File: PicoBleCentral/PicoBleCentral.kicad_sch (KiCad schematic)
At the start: 10 parts, among them IC2 VREG-OKI-78SR-3.3/1.5-W36, J5 Sel Vreg In, Q3 DMG2305UX-7, U2 R-78E5.0-1.0

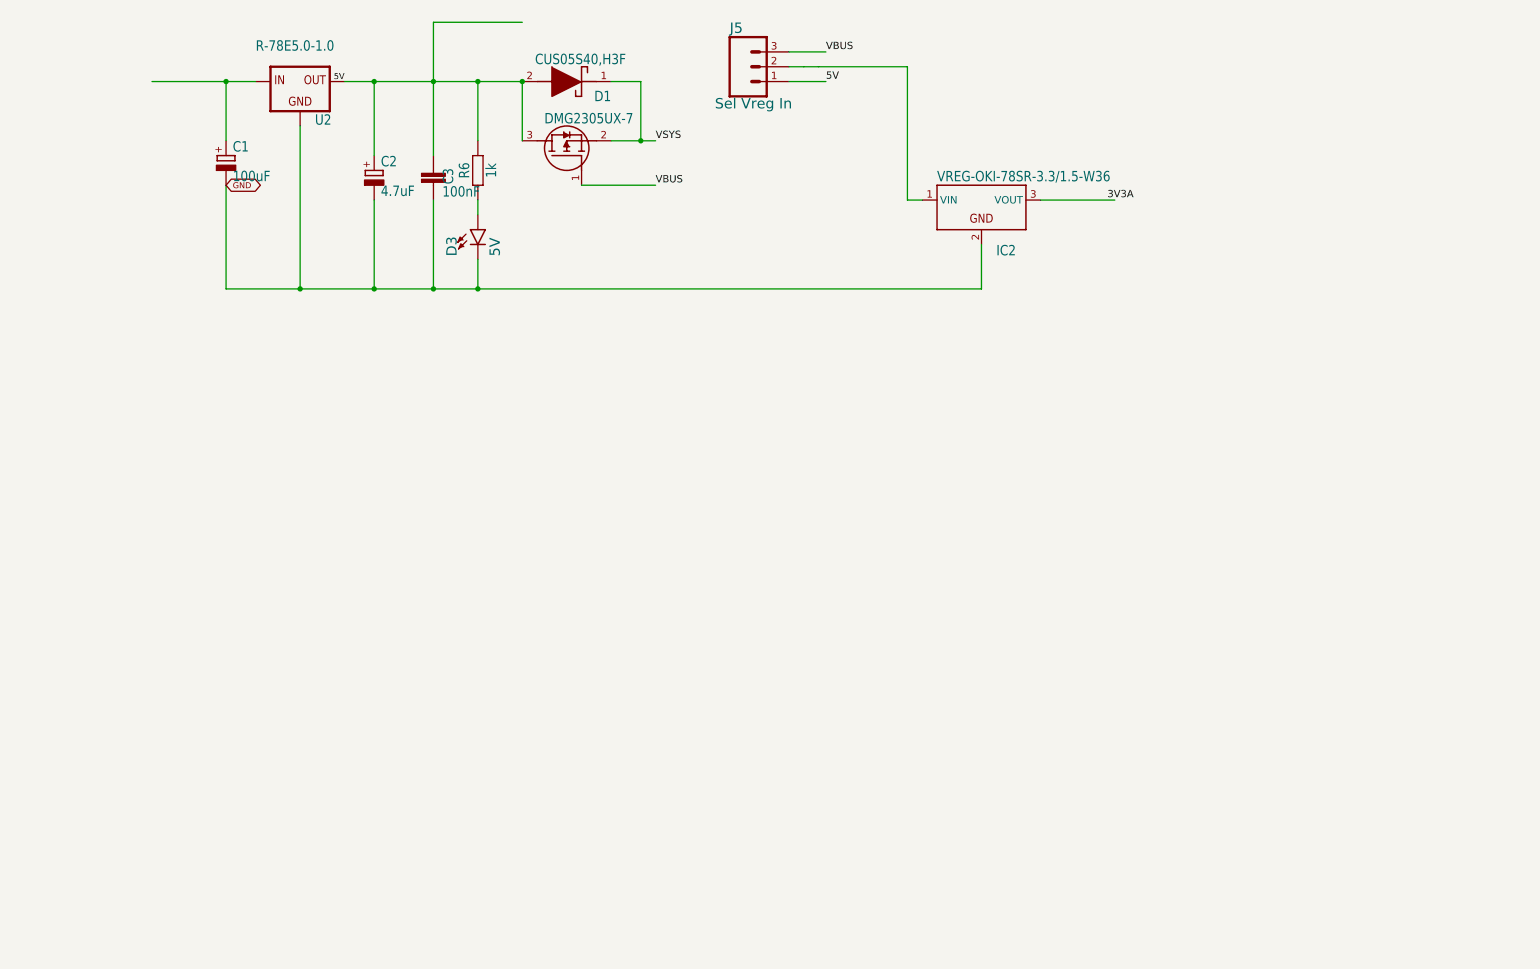
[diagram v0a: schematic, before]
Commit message: 26/05/25 20:18 Titan.local
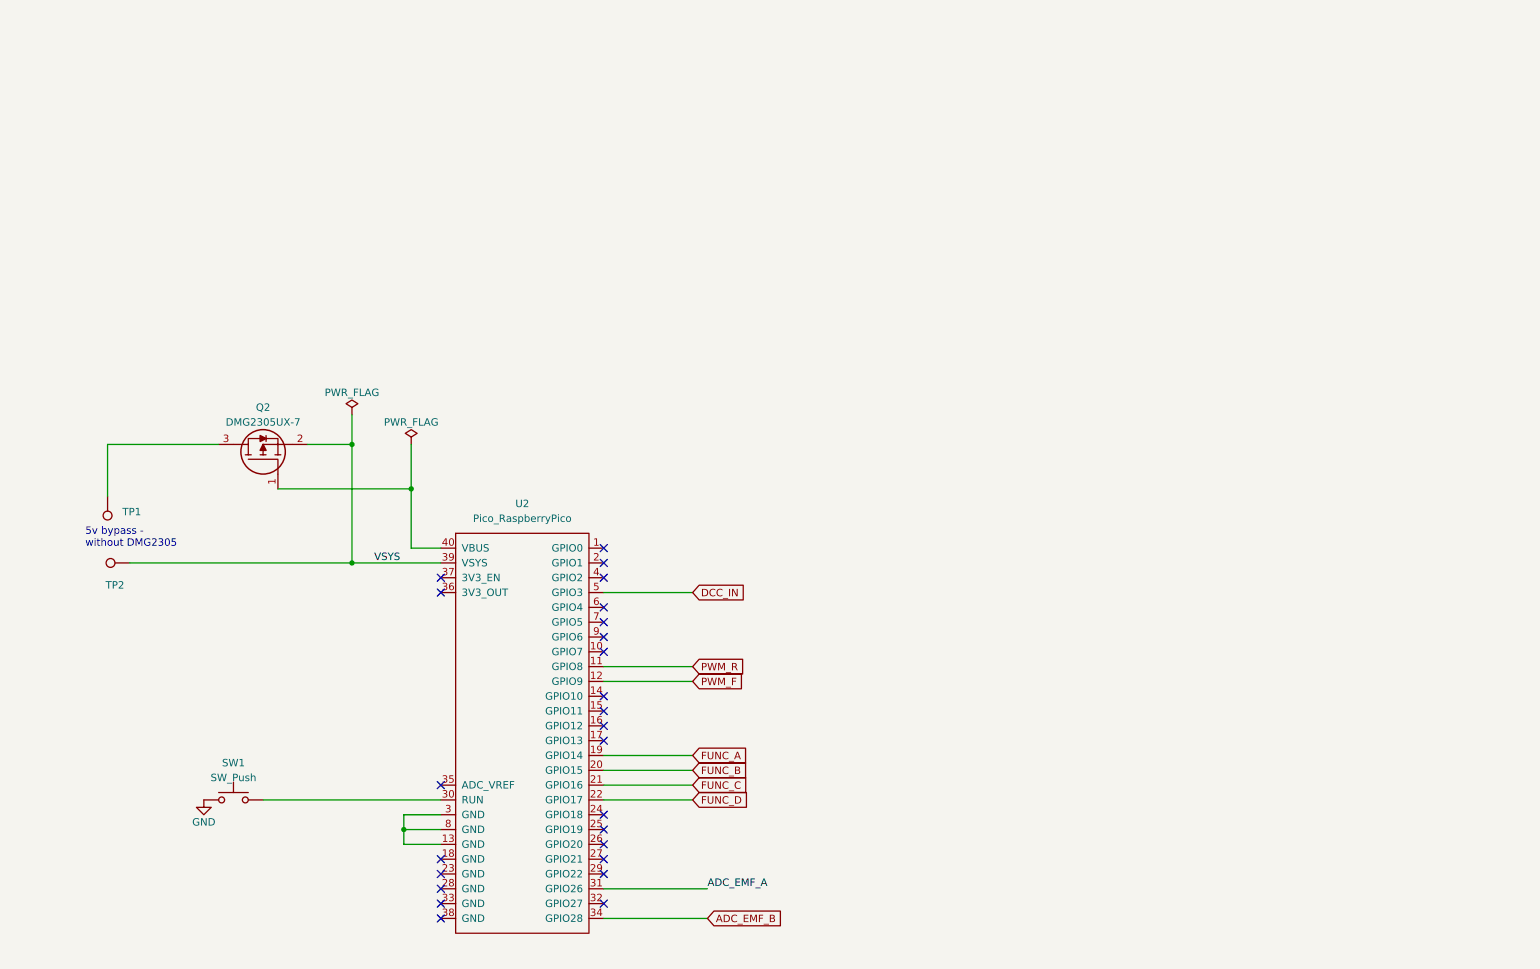
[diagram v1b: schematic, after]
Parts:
- removed C1: 100uF, PicoCanSmd31:E5-8,5, symbol PicoCanSmd31-eagle-import:CPOL-EUE5-8.5
- removed C2: 4.7uF, PicoCanSmd31:E5-8,5, symbol PicoCanSmd31-eagle-import:CPOL-EUE5-8.5
- removed C3: 100nF, PicoCanSmd31:C025-024X044, symbol PicoCanSmd31-eagle-import:C-EU025-024X044
- removed D1: CUS05S40,H3F, PicoCanSmd31:1SS357TPH3F, symbol PicoCanSmd31-eagle-import:CUS05S40,H3F
- removed D3: 5V, PicoCanSmd31:LED_3MM, symbol PicoCanSmd31-eagle-import:LED3MM
- removed IC2: VREG-OKI-78SR-3.3/1.5-W36, PicoCanSmd31:OKI-78SR, symbol PicoCanSmd31-eagle-import:VREG-OKI-78SR-3.3/1.5-W36
- removed J5: Sel Vreg In, PicoCanSmd31:1X03, symbol PicoCanSmd31-eagle-import:CONN_03
- removed Q3: DMG2305UX-7, PicoCanSmd31:SOT96P240X110-3N, symbol PicoCanSmd31-eagle-import:DMG2305UX-7
- removed R6: 1k, PicoCanSmd31:C1206, symbol PicoCanSmd31-eagle-import:RESISTOR-1206
- removed U2: R-78E5.0-1.0, PicoCanSmd31:DC-DC_CONVERTER_78XX, symbol PicoCanSmd31-eagle-import:R-78E5.0-1.0
- added Q2: DMG2305UX-7, Package_TO_SOT_SMD:SOT-23-3, symbol DMG2305UX-7:DMG2305UX-7
- added SW1: SW_Push, Button_Switch_SMD:SW_Tactile_SPST_NO_Straight_CK_PTS636Sx25SMTRLFS, symbol Switch:SW_Push
- added TP1, TP2: TestPoint, TestPoint:TestPoint_Pad_2.0x2.0mm, symbol Connector:TestPoint
- added U2: Pico_RaspberryPico, PicoNoSwd:RaspberryPico_TH_NoSWD, symbol PicoNoSwd:RaspberryPico-Pico
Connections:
- net GND: now also SW1.2
- net VSYS: now also Q2.2, TP2.1, U2.39 (VSYS)
- new net: Q2.1, U2.40 (VBUS)
- new net: Q2.3, TP1.1
- new net: SW1.1, U2.30 (RUN)
- new net: U2.13 (GND), U2.3 (GND), U2.8 (GND)
- new net ADC_EMF_A: U2.31 (GPIO26)
- new net ADC_EMF_B: U2.34 (GPIO28)
- new net DCC_IN: U2.5 (GPIO3)
- new net FUNC_A: U2.19 (GPIO14)
- new net FUNC_B: U2.20 (GPIO15)
- new net FUNC_C: U2.21 (GPIO16)
- new net FUNC_D: U2.22 (GPIO17)
- new net PWM_F: U2.12 (GPIO9)
- new net PWM_R: U2.11 (GPIO8)
- no-connect marks 0 -> 25
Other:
- note added: "5v bypass - without DMG2305"

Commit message: 26/05/25 20:40 Titan.local
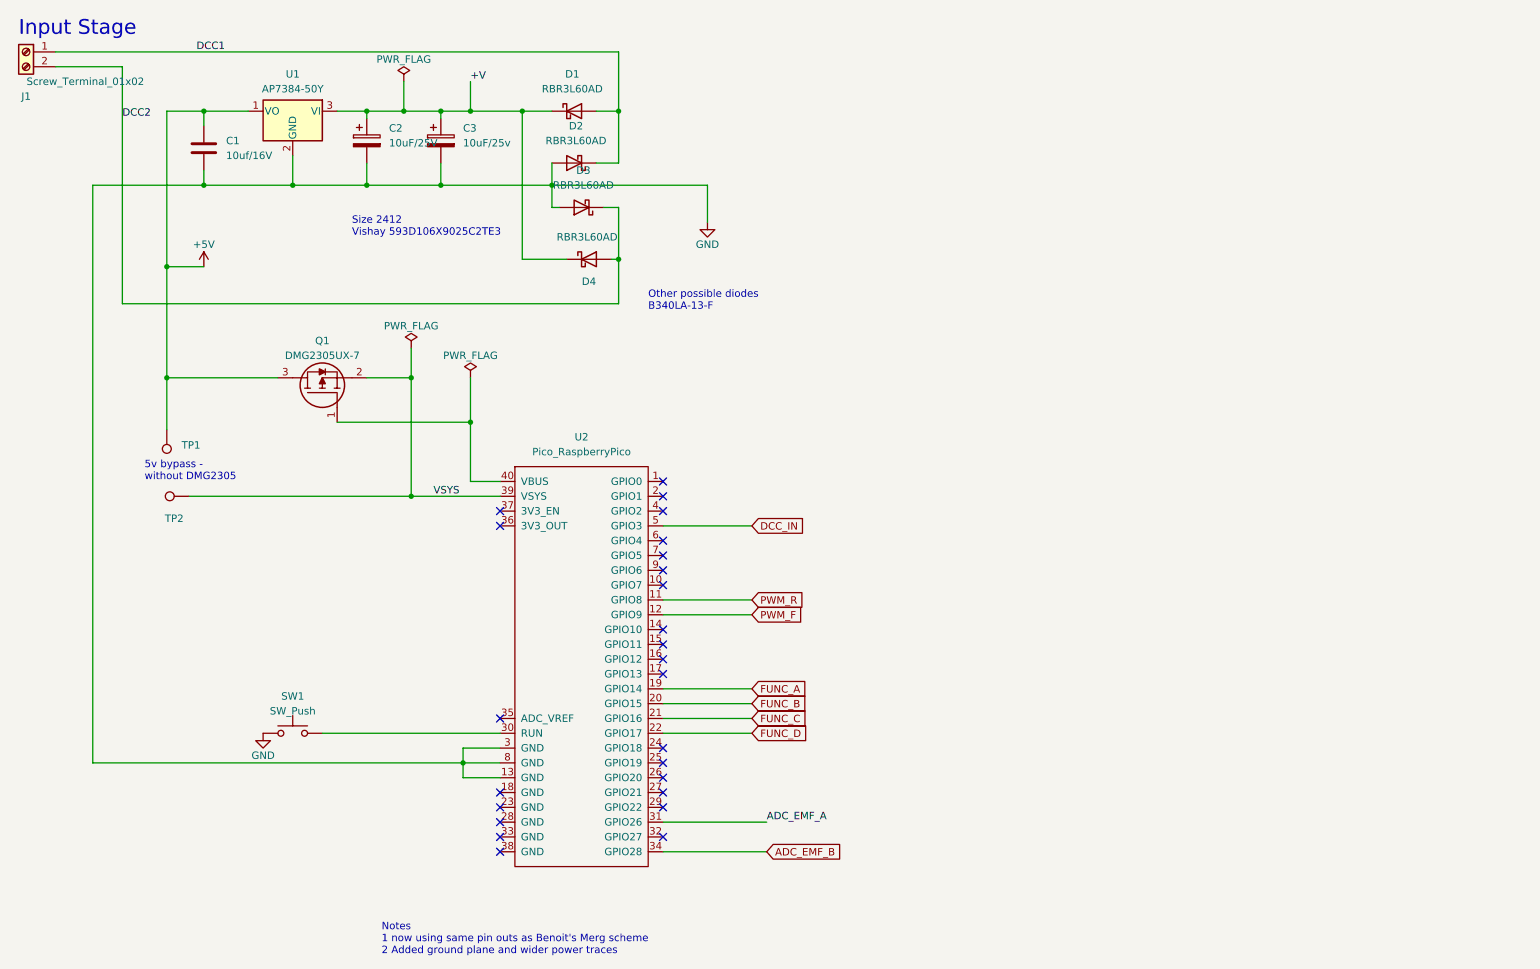
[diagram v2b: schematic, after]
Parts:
- removed Q2: DMG2305UX-7, Package_TO_SOT_SMD:SOT-23-3, symbol DMG2305UX-7:DMG2305UX-7
- added C1: 10uf/16V, Capacitor_SMD:C_1206_3216Metric_Pad1.33x1.80mm_HandSolder, symbol Device:C
- added C2: 10uF/25V, Capacitor_Tantalum_SMD:CP_EIA-6032-20_AVX-F_Pad2.25x2.35mm_HandSolder, symbol Device:C_Polarized
- added C3: 10uF/25v, Capacitor_Tantalum_SMD:CP_EIA-6032-20_AVX-F_Pad2.25x2.35mm_HandSolder, symbol Device:C_Polarized
- added D1, D2, D3, D4: RBR3L60AD, Diode_SMD:D_SMA_Handsoldering, symbol Device:D_Schottky
- added J1: Screw_Terminal_01x02, TerminalBlock_Phoenix:TerminalBlock_Phoenix_PT-1,5-2-3.5-H_1x02_P3.50mm_Horizontal, symbol Connector:Screw_Terminal_01x02
- added Q1: DMG2305UX-7, Package_TO_SOT_SMD:SOT-23-3, symbol DMG2305UX-7:DMG2305UX-7
- added U1: AP7384-50Y, Package_TO_SOT_SMD:SOT-89-3, symbol Regulator_Linear:AP7384-50Y
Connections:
- net GND: now also U2.13 (GND), U2.3 (GND), U2.8 (GND), C1.2, C2.2, C3.2, D2.2 (A), D3.2 (A), U1.2 (GND)
- net VSYS: now also Q1.2
- net at U2.40 (VBUS): now also Q1.1
- net +5V: now reaches TP1.1
- net +5V: now also C1.1, Q1.3, U1.1 (VO)
- new net +V: C2.1, C3.1, D1.1 (K), D4.1 (K), U1.3 (VI)
- new net DCC1: D1.2 (A), D2.1 (K), J1.1 (Pin_1)
- new net DCC2: D3.1 (K), D4.2 (A), J1.2 (Pin_2)
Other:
- note added: "Input Stage"
- note added: "Notes 1 now using same pin outs as Benoit's Merg scheme 2 Added ground plane and wider power traces"
- note added: "Other possible diodes B340LA-13-F"
- note added: "Size 2412 Vishay 593D106X9025C2TE3"
- title: (none) -> DCC Decoder 4a - modified PCB - As 4 but with ground plane

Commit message: 26/05/25 22:33 Titan.local
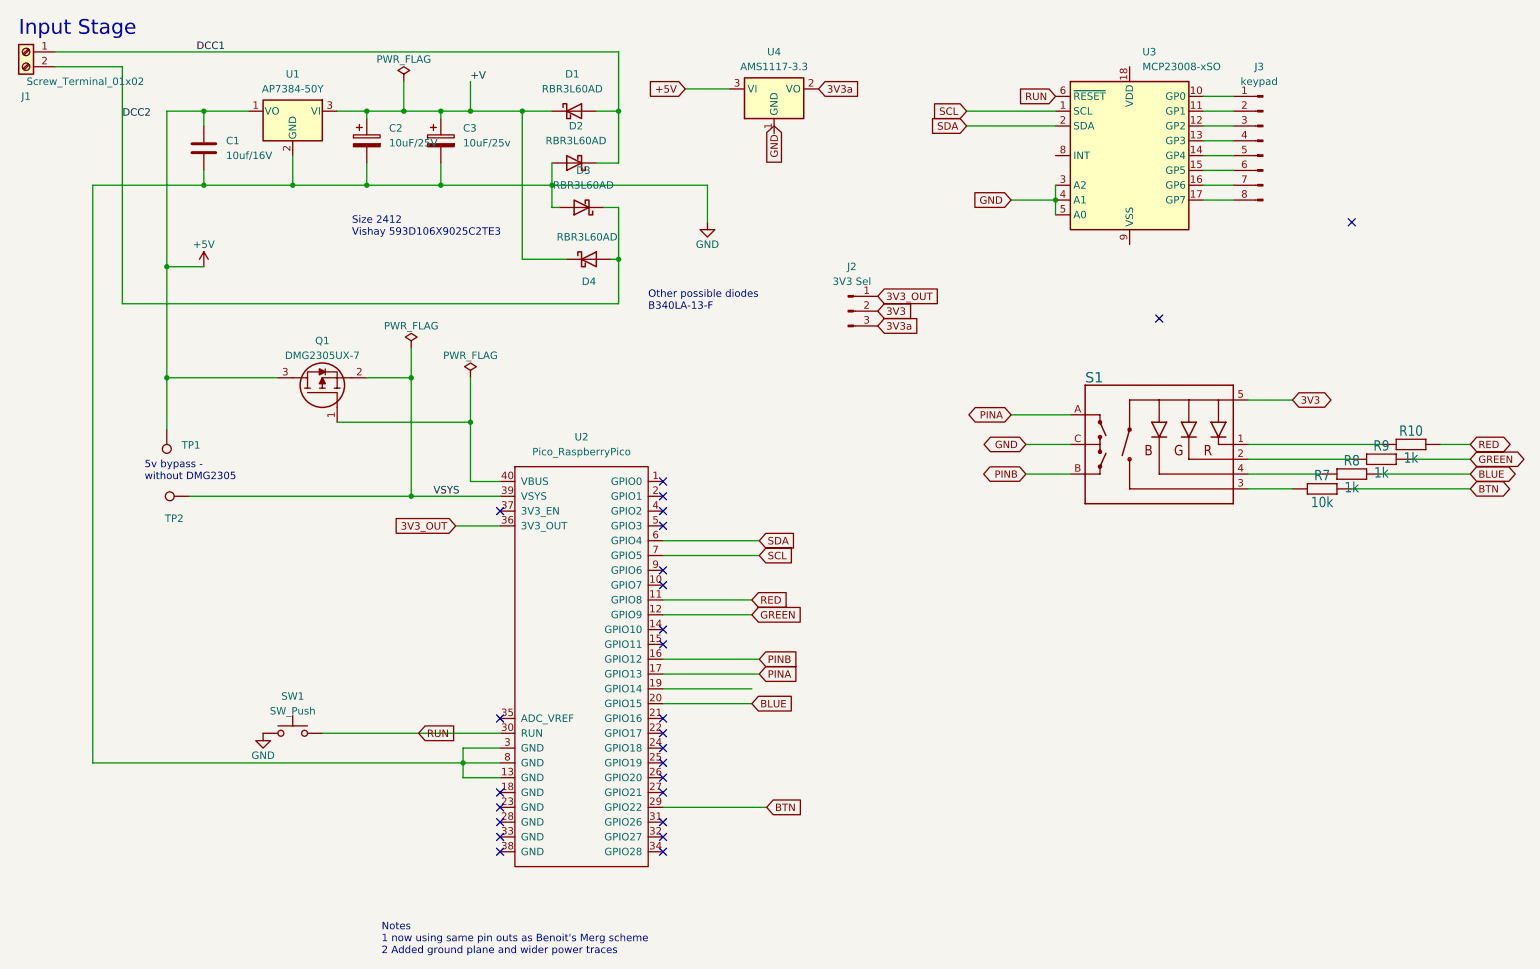
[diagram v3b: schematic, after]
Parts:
- added J2: 3V3 Sel, Connector_PinHeader_2.54mm:PinHeader_1x03_P2.54mm_Vertical, symbol Connector:Conn_01x03_Pin
- added J3: keypad, Connector_PinHeader_2.54mm:PinHeader_1x08_P2.54mm_Vertical, symbol Connector:Conn_01x08_Pin
- added R10, R8, R9: 1k, Resistor_SMD:R_1206_3216Metric_Pad1.30x1.75mm_HandSolder, symbol PicoCanSmd31-eagle-import:RESISTOR-1206
- added R7: 10k, Resistor_SMD:R_1206_3216Metric_Pad1.30x1.75mm_HandSolder, symbol PicoCanSmd31-eagle-import:RESISTOR-1206
- added S1: ENCODER-RGB-SWITCH, Sparkfun switch:ENCODER_LED_3_KIT, symbol PicoCanSmd31-eagle-import:ENCODER-RGB-SWITCH
- added U3: MCP23008-xSO, Package_SO:SOIC-18W_7.5x11.6mm_P1.27mm, symbol Interface_Expansion:MCP23008-xSO
- added U4: AMS1117-3.3, Package_TO_SOT_SMD:SOT-223-3_TabPin2, symbol Regulator_Linear:AMS1117-3.3
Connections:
- net +5V: now also U4.3 (VI)
- net GND: now also S1.C, U3.3 (A2), U3.4 (A1), U3.5 (A0)
- net PINB: now reaches U2.16 (GPIO12)
- net PINB: now also S1.B
- net PINA: now reaches U2.17 (GPIO13)
- net PINA: now also S1.A
- net BTN: now reaches U2.29 (GPIO22)
- net BTN: now also R7.2
- net RUN: now reaches SW1.1, U2.30 (RUN)
- net RUN: now also U3.6 (~{RESET})
- net 3V3_OUT: now reaches U2.36 (3V3_OUT)
- net 3V3_OUT: now also J2.1 (Pin_1)
- net SDA: now reaches U2.6 (GPIO4)
- net SDA: now also U3.2 (SDA)
- net SCL: now reaches U2.7 (GPIO5)
- net SCL: now also U3.1 (SCL)
- net ADC_EMF_A: no longer names the net of U2.31 (GPIO26)
- net ADC_EMF_B: no longer names the net of U2.34 (GPIO28)
- net DCC_IN: no longer names the net of U2.5 (GPIO3)
- net FUNC_A: no longer names the net of U2.19 (GPIO14)
- net FUNC_B renamed BLUE
- net BLUE: now also R8.2
- net FUNC_C: no longer names the net of U2.21 (GPIO16)
- net FUNC_D: no longer names the net of U2.22 (GPIO17)
- net PWM_F renamed GREEN
- net GREEN: now also R9.2
- net PWM_R renamed RED
- net RED: now also R10.2
- new net: R10.1, S1.1 (-R)
- new net: R9.1, S1.2 (-G)
- new net: R7.1, S1.3 (SW)
- new net: R8.1, S1.4 (-B)
- new net: J3.1 (Pin_1), U3.10 (GP0)
- new net: J3.2 (Pin_2), U3.11 (GP1)
- new net: J3.3 (Pin_3), U3.12 (GP2)
- new net: J3.4 (Pin_4), U3.13 (GP3)
- new net: J3.5 (Pin_5), U3.14 (GP4)
- new net: J3.6 (Pin_6), U3.15 (GP5)
- new net: J3.7 (Pin_7), U3.16 (GP6)
- new net: J3.8 (Pin_8), U3.17 (GP7)
- new net 3V3: J2.2 (Pin_2), S1.5 (+)
- new net 3V3a: J2.3 (Pin_3), U4.2 (VO)
- no-connect marks 25 -> 26
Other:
- title: DCC Decoder 4a - modified PCB - As 4 but with ground plane -> Pico Ble Central for loco 
